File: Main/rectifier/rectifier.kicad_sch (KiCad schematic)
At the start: 17 parts, among them J1 Screw_Terminal_01x04, J2 Jack-DC, J3 Screw_Terminal_01x02, Q1 BS170, U1 ESP32-C3-WROOM-02, U2 LM2596S-5, U3 HC-SR04, U4 DM-OLED096-636, U5 SIM7000E

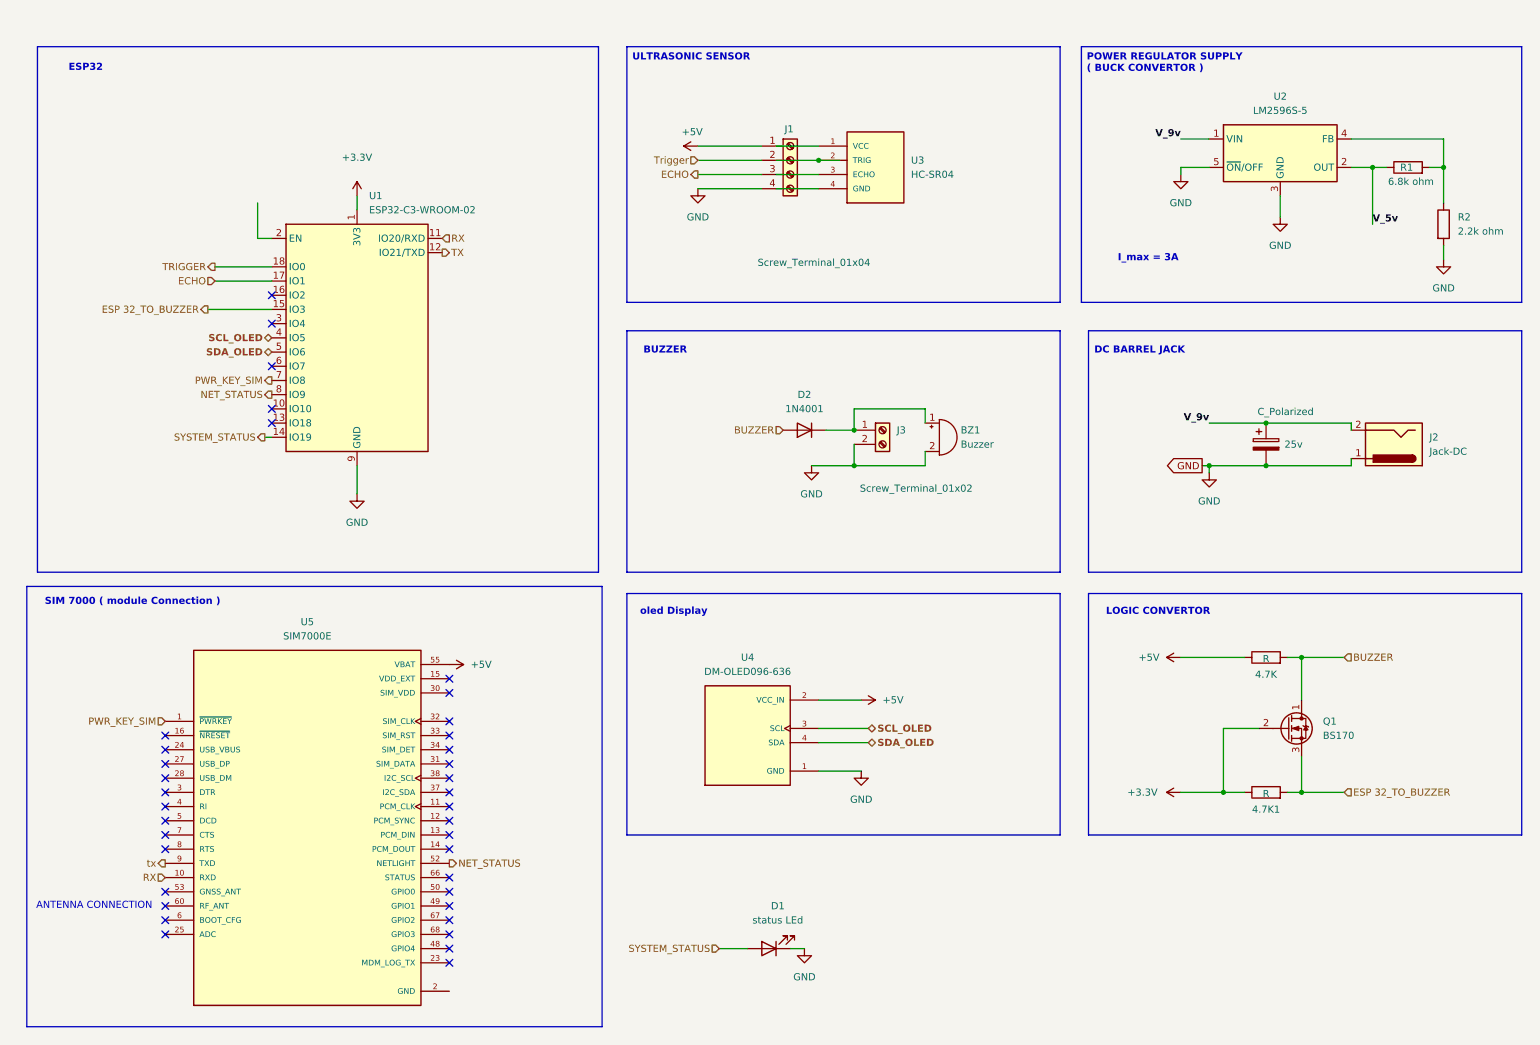
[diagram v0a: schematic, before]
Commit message: updated schematic
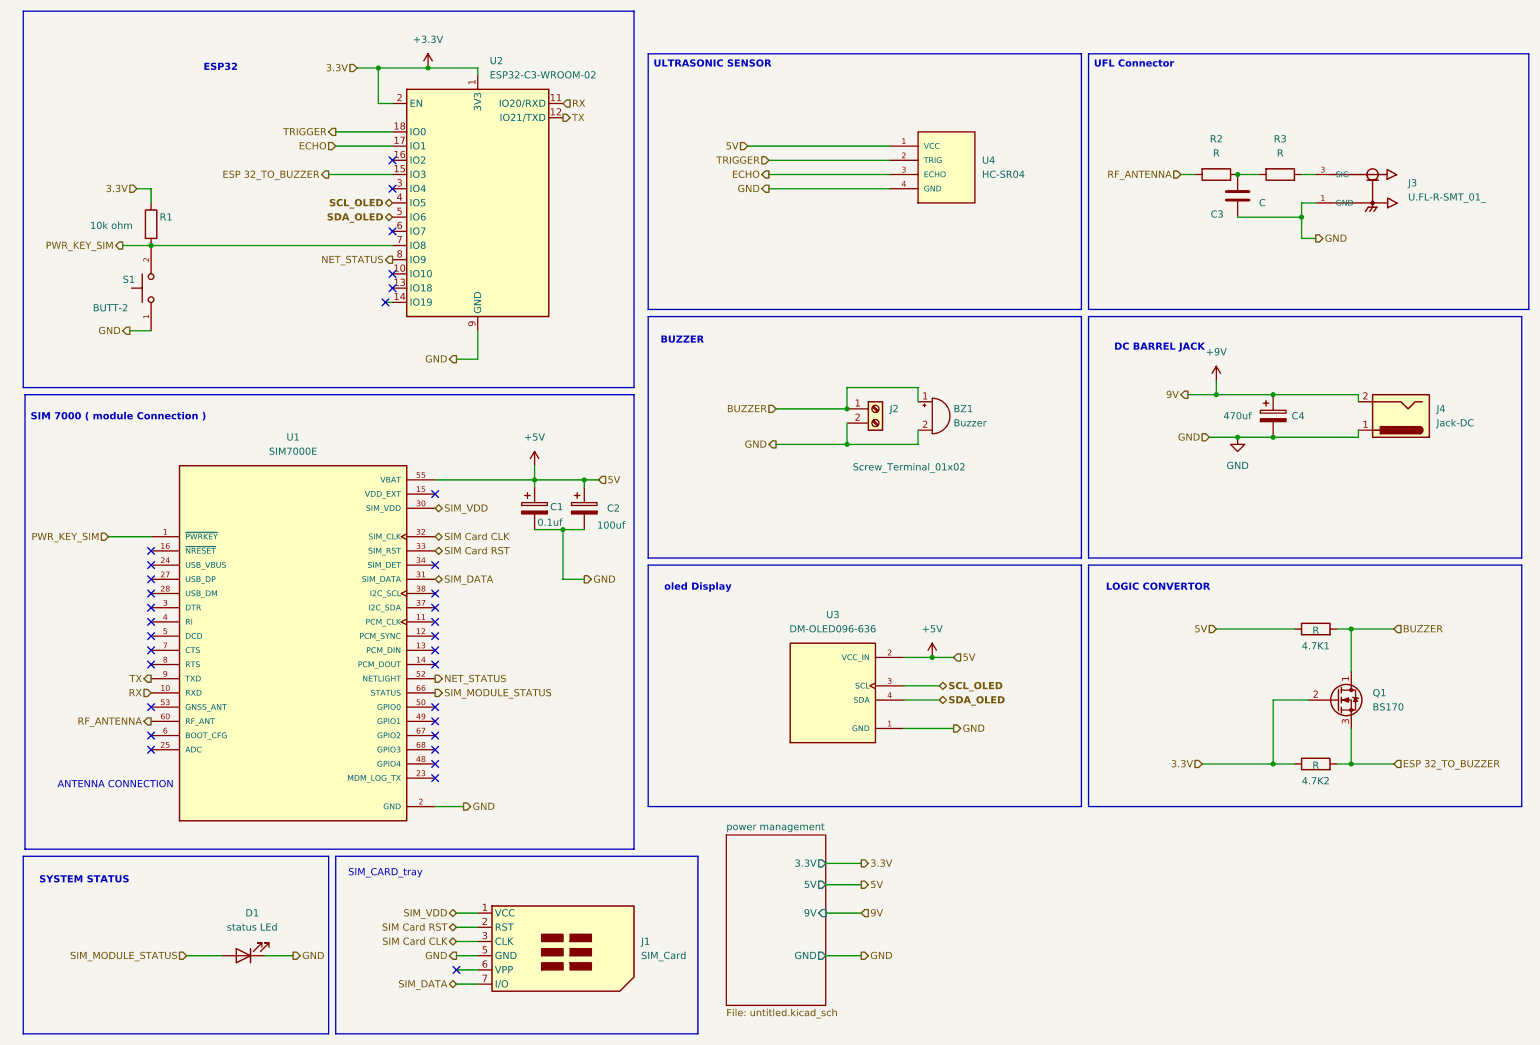
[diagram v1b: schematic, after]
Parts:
- removed D2: 1N4001, Diode_THT:D_DO-41_SOD81_P10.16mm_Horizontal, symbol Diode:1N4001
- removed J1: Screw_Terminal_01x04, symbol Connector:Screw_Terminal_01x04
- removed U2: LM2596S-5, Package_TO_SOT_SMD:TO-263-5_TabPin3, symbol Regulator_Switching:LM2596S-5
- added C1: 0.1uf, Capacitor_Tantalum_SMD:CP_EIA-1608-08_AVX-J_HandSolder, symbol Device:C_Polarized
- added C2: 100uf, Capacitor_Tantalum_SMD:CP_EIA-1608-08_AVX-J_HandSolder, symbol Device:C_Polarized
- added C3: C, Capacitor_SMD:C_0402_1005Metric_Pad0.74x0.62mm_HandSolder, symbol Device:C
- added J1: SIM_Card, Connector_JAE:JAE_SIM_Card_SF72S006, symbol Connector:SIM_Card
- added J3: U.FL-R-SMT_01_, U.FL-R-SMT_01_:HRS_U.FL-R-SMT_01_, symbol U.FL-R-SMT_01_:U.FL-R-SMT_01_
- added R3: R, Resistor_SMD:R_0402_1005Metric, symbol Device:R
- added S1: BUTT-2, BUTT-2:SW_BUTT-2, symbol PUSH_BUTT-2:BUTT-2
- BZ1: footprint (none) -> Buzzer_Beeper:Buzzer_TDK_PS1240P02BT_D12.2mm_H6.5mm
- C4: renamed from 25v; value C_Polarized -> 470uf
- J4: renamed from J2; footprint (none) -> Connector_BarrelJack:BarrelJack_GCT_DCJ200-10-A_Horizontal
- R1: value 6.8k ohm -> 10k ohm; footprint Resistor_THT:R_Box_L13.0mm_W4.0mm_P9.00mm -> Resistor_SMD:R_0402_1005Metric
- R2: value 2.2k ohm -> R; footprint Resistor_THT:R_Box_L13.0mm_W4.0mm_P9.00mm -> Resistor_SMD:R_0402_1005Metric
- renumbered 4.7K to 4.7K1, 4.7K1 to 4.7K2, J3 to J2, U5 to U1, U1 to U2, U4 to U3, U3 to U4
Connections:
- net V_5v is gone; now on net +3.3V: R1.1
- net tx is gone; now on net TX: U1.9 (TXD)
- net +3.3V: now also U2.2 (EN)
- net +5V: now also U4.1 (VCC), C1.1, C2.1
- net BUZZER: now also BZ1.1 (+), J2.1 (Pin_1)
- net ECHO: now also U4.3 (ECHO)
- net GND: now also U4.4 (GND), C1.2, C2.2, C3.2, J1.5 (GND), J3.1 (GND), J3.2 (GND), S1.1; no longer R2.2
- net PWR_KEY_SIM: now also R1.2, S1.2
- net TRIGGER: now also U4.2 (TRIG)
- net at R2.1: now also C3.1, R3.2; no longer R1.2
- net SIM_VDD: now reaches U1.30 (SIM_VDD)
- net SIM_VDD: now also J1.1 (VCC)
- net SIM_DATA : now reaches U1.31 (SIM_DATA)
- net SIM_DATA : now also J1.7 (I/O)
- net SIM Card CLK: now reaches U1.32 (SIM_CLK)
- net SIM Card CLK: now also J1.3 (CLK)
- net SIM Card RST: now reaches U1.33 (SIM_RST)
- net SIM Card RST: now also J1.2 (RST)
- net RF_ANTENNA: now reaches U1.60 (RF_ANT)
- net RF_ANTENNA: now also R2.2
- net SIM_MODULE_STATUS: now reaches U1.66 (STATUS)
- net SIM_MODULE_STATUS: now also D1.2 (A)
- net SYSTEM_STATUS: no longer names the net of U2.14 (IO19)
- net SYSTEM_STATUS: no longer D1.2 (A)
- net V_9v renamed +9V
- new net: J3.3 (SIG), R3.1
- no-connect marks 37 -> 33
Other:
- added sheet power management (untitled.kicad_sch)
- note added: "SIM_CARD_tray"
- note added: "SYSTEM STATUS"
- note removed: "I_max = 3A"
- moved on the sheet: 4.7K1, 4.7K2, BZ1, C4, D1, J2, J4, Q1, U1, U2, U3, U4
